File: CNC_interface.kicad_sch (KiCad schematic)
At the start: 26 parts, among them J1 Conn_01x04_Male, J10 Conn_01x08, J11 Conn_01x08, J12 Conn_01x08, J13 Conn_01x08, J14 Conn_01x03_Male, J15 Conn_01x03_Male, J16 Conn_01x03_Male, J17 Conn_01x08, J18 Conn_01x10, J2 Conn_01x04_Male, J3 Conn_01x04_Male, J5 Screw_Terminal_01x02, J6 Screw_Terminal_01x02, J8 Conn_01x08, J9 Conn_01x08, Q1 Q_NMOS_GDS, U4 LM2596S-5

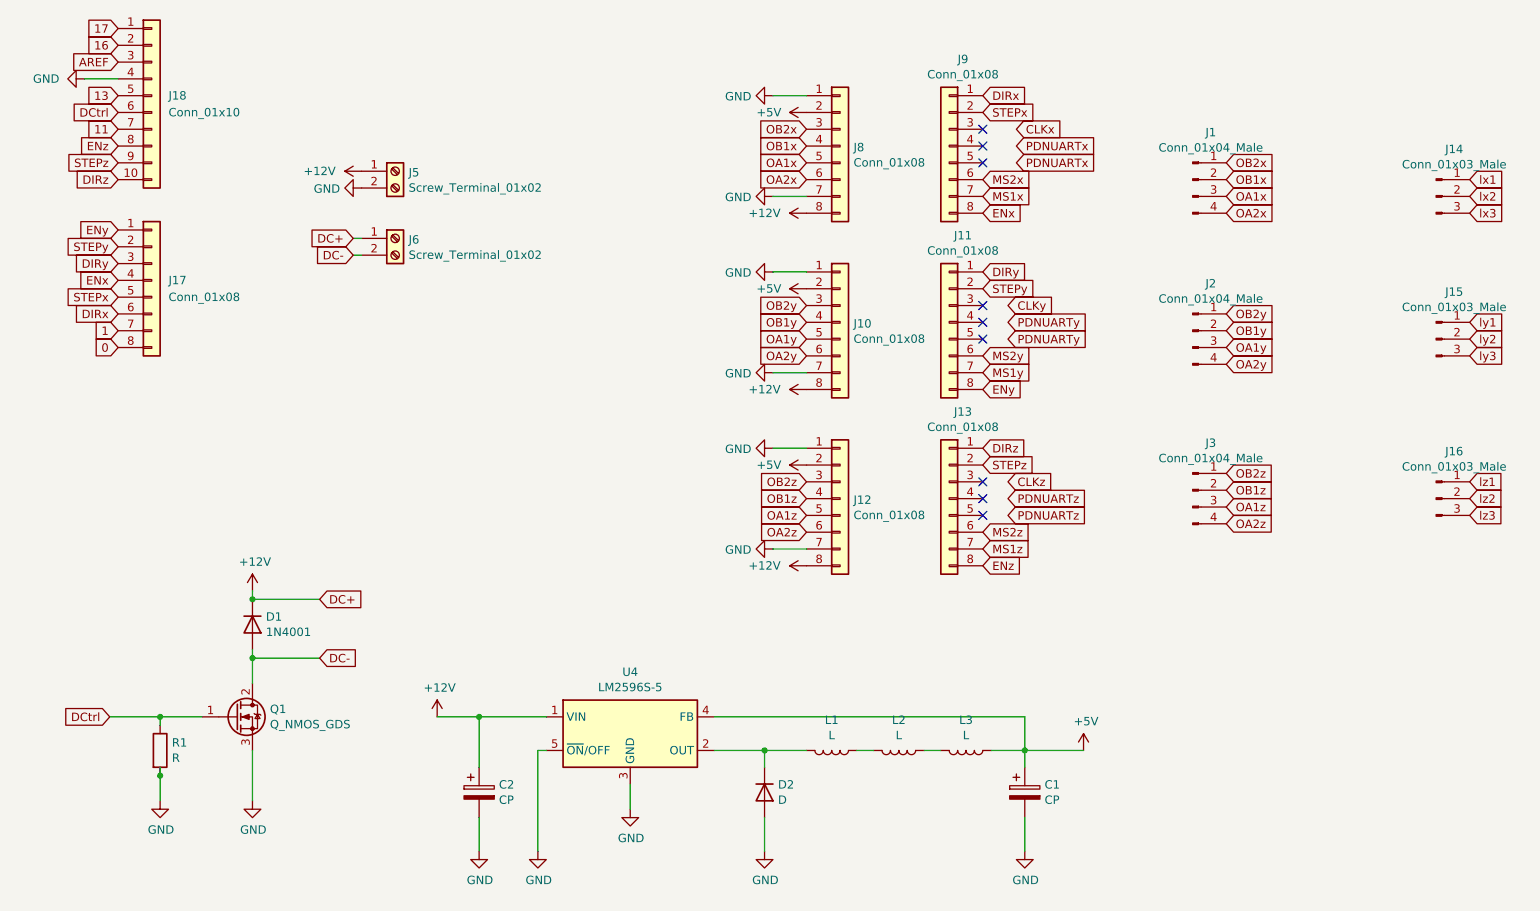
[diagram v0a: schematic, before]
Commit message: debut seance
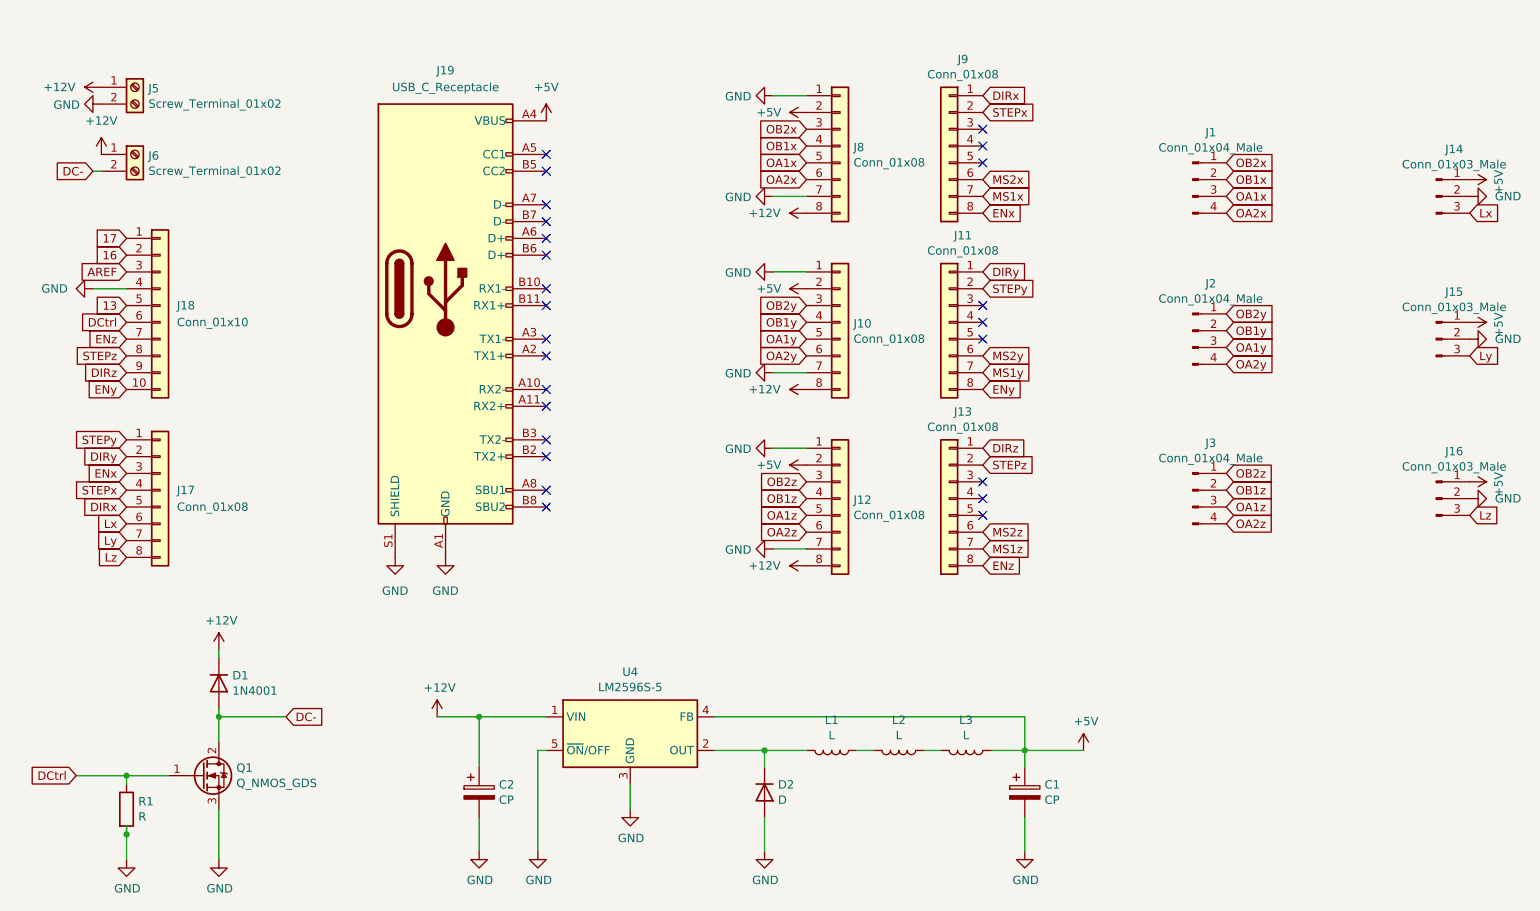
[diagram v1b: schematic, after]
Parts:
- added J19: USB_C_Receptacle, Connector_USB:USB_C_Receptacle_Amphenol_12401548E4-2A_CircularHoles, symbol Connector:USB_C_Receptacle
- D2: footprint (none) -> Diode_THT:D_DO-201AD_P15.24mm_Horizontal
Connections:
- net 11 is gone; now on net ENz: J18.7 (Pin_7)
- net lx1 is gone; now on net +5V: J14.1 (Pin_1)
- net lx2 is gone; now on net GND: J14.2 (Pin_2)
- net ly1 is gone; now on net +5V: J15.1 (Pin_1)
- net ly2 is gone; now on net GND: J15.2 (Pin_2)
- net ly3 is gone; now on net Ly: J15.3 (Pin_3)
- net lz1 is gone; now on net +5V: J16.1 (Pin_1)
- net lz2 is gone; now on net GND: J16.2 (Pin_2)
- net lz3 is gone; now on net Lz: J16.3 (Pin_3)
- net +5V: now also J19.A4 (VBUS), J19.A9 (VBUS), J19.B4 (VBUS), J19.B9 (VBUS)
- net DIRx: now also J17.5 (Pin_5); no longer J17.6 (Pin_6)
- net DIRy: now also J17.2 (Pin_2); no longer J17.3 (Pin_3)
- net DIRz: now also J18.9 (Pin_9); no longer J18.10 (Pin_10)
- net ENx: now also J17.3 (Pin_3); no longer J17.4 (Pin_4)
- net ENy: now also J18.10 (Pin_10); no longer J17.1 (Pin_1)
- net ENz: no longer J18.8 (Pin_8)
- net GND: now also J19.A1 (GND), J19.A12 (GND), J19.B1 (GND), J19.B12 (GND), J19.S1 (SHIELD)
- net STEPx: now also J17.4 (Pin_4); no longer J17.5 (Pin_5)
- net STEPy: now also J17.1 (Pin_1); no longer J17.2 (Pin_2)
- net STEPz: now also J18.8 (Pin_8); no longer J18.9 (Pin_9)
- net 0 renamed Lz
- net 1 renamed Ly
- net lx3 renamed Lx
- net Lx: now also J17.6 (Pin_6)
- no-connect marks 9 -> 25
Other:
- moved on the sheet: D1, J17, J18, J5, J6, Q1, R1
